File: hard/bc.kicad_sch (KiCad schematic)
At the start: 1 part

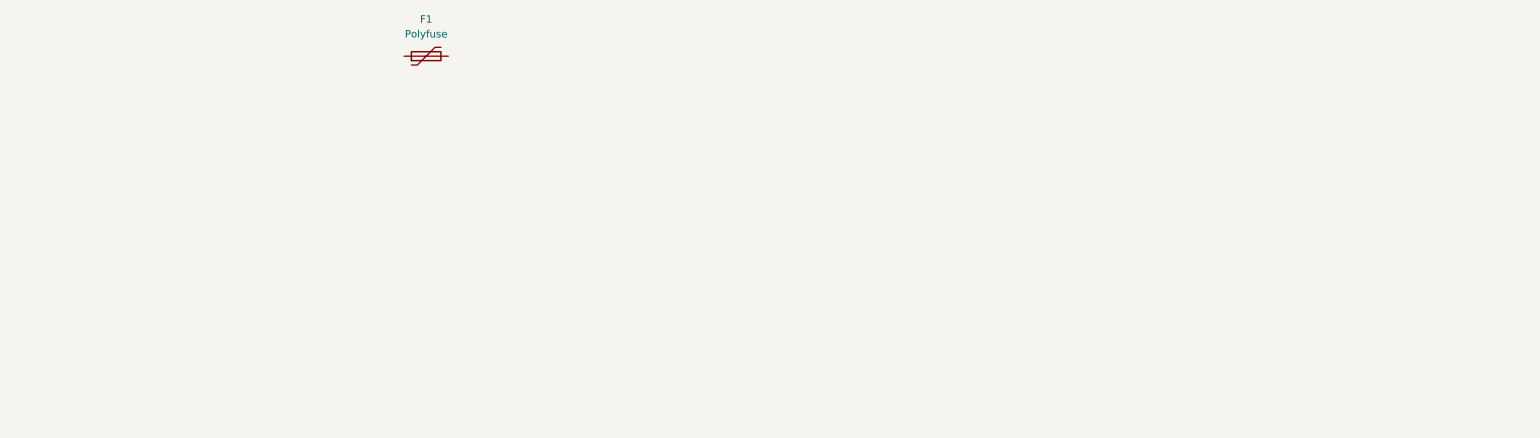
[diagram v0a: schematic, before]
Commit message: edit
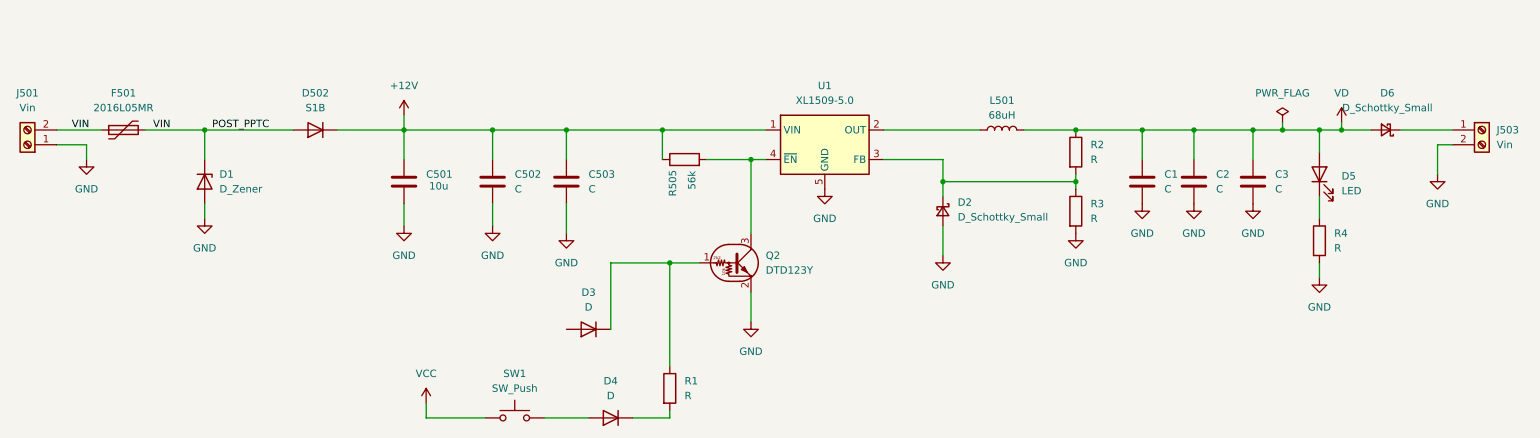
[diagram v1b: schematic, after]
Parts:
- added C1, C2, C3, C502, C503: C, symbol Device:C
- added C501: 10u, symbol Device:C
- added D1: D_Zener, symbol Device:D_Zener
- added D2, D6: D_Schottky_Small, symbol Device:D_Schottky_Small
- added D3, D4: D, symbol Device:D
- added D5: LED, symbol Device:LED
- added D502: S1B, symbol Device:D
- added J501, J503: Vin, symbol Connector:Screw_Terminal_01x02
- added L501: 68uH, symbol Device:L
- added Q2: DTD123Y, symbol Transistor_BJT:DTD123Y
- added R1, R2, R3, R4: R, symbol Device:R
- added R505: 56k, symbol Device:R
- added SW1: SW_Push, symbol Switch:SW_Push
- added U1: XL1509-5.0, Package_SO:SOIC-8_3.9x4.9mm_P1.27mm, symbol Regulator_Switching:XL1509-5.0
- F501: renamed from F1; value Polyfuse -> 2016L05MR
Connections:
- net POST_PPTC: now reaches F501.1
- net POST_PPTC: now also F501.2, D1.1 (K), D502.2 (A), J501.2 (Pin_2)
- new net: D5.1 (K), R4.1
- new net: D3.1 (K), Q2.1 (B), R1.1
- new net: D4.1 (K), R1.2
- new net: D2.1 (K), R2.2, R3.1, U1.3 (FB)
- new net: Q2.3 (C), R505.2, U1.4 (~{EN})
- new net: D4.2 (A), SW1.2
- new net: L501.1, U1.2 (OUT)
- new net: D6.1 (K), J503.1 (Pin_1)
- new net +12V: C501.1, C502.1, C503.1, D502.1 (K), R505.1, U1.1 (VIN)
- new net GND: C1.2, C2.2, C3.2, C501.2, C502.2, C503.2, D1.2 (A), D2.2 (A), J501.1 (Pin_1), J503.2 (Pin_2), Q2.2 (E), R3.2, R4.2, U1.5 (GND), U1.6 (GND), U1.7 (GND), U1.8 (GND)
- new net VCC: SW1.1
- new net VD: C1.1, C2.1, C3.1, D5.2 (A), D6.2 (A), L501.2, R2.1
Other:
- moved on the sheet: F501
